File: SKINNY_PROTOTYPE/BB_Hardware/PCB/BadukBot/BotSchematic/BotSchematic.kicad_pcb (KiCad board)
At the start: 2 copper layers, 68 parts, among them J1 MOLEX_78171-0002, J2 MOLEX_78171-0003, Q1 MMBT3904LT1G, Q2 MMBT3904LT1G, Q3 MMBT3904LT1G, Q4 MMBT3904LT1G, U1 STM32F051C8U6, U2 LSM6DS3, U3 A3901SEJTR-T, U4 ADP122ACPZ-3.3-R7, U5 AT42QT1070-MMHCT-ND, U6 MCP73831T-2ACI_OT, U7 NRF24L01P-R7, Y1 7V-16.000MAAE-T

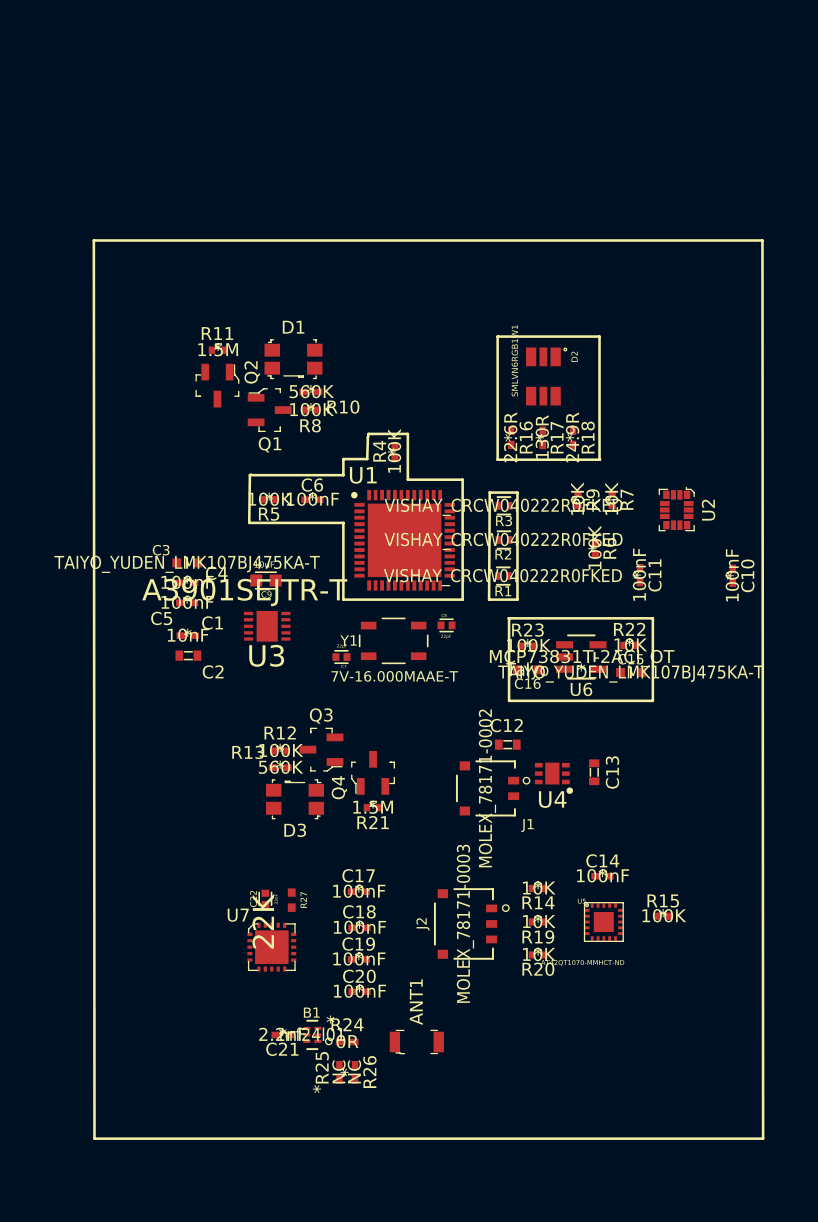
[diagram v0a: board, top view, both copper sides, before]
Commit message: PCB adjustments
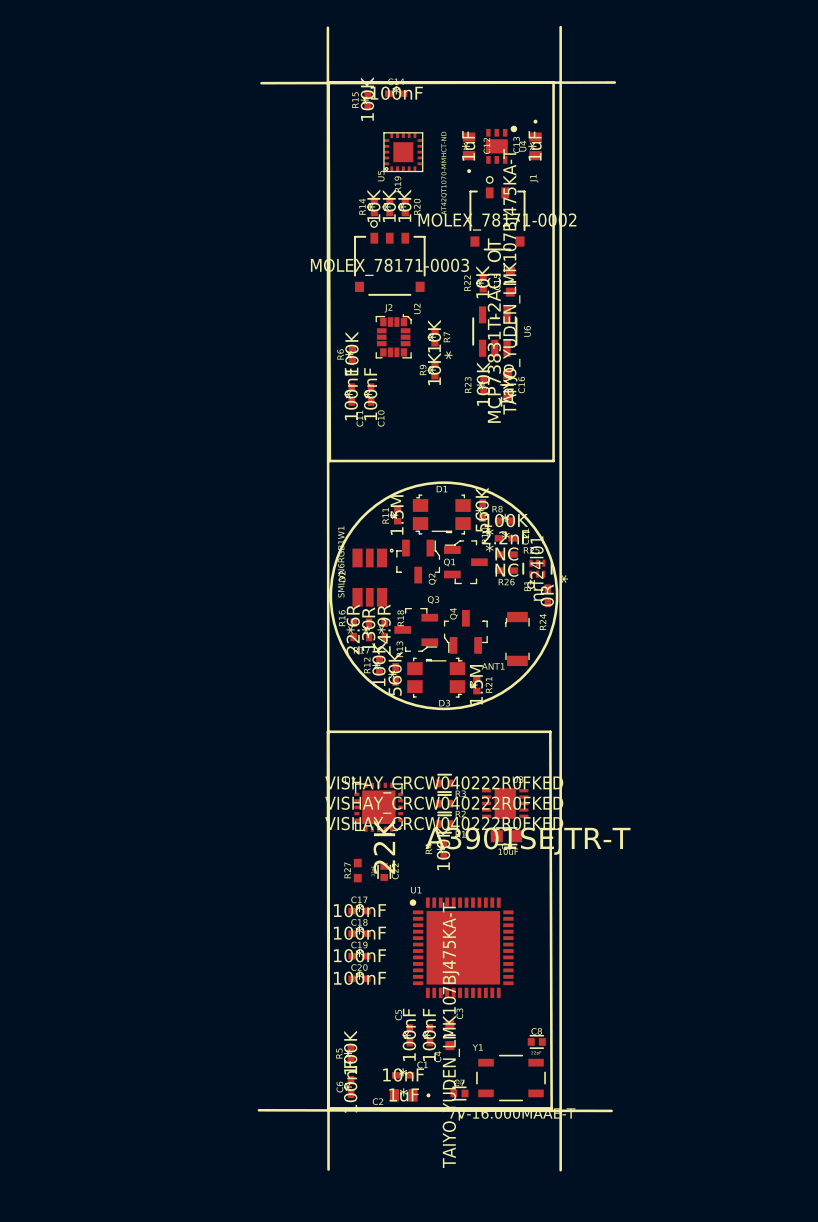
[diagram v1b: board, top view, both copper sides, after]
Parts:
- B1: footprint 2450BM14A0002T:JOHANSON_2450BM14A0002T_0 -> JOHANSON_2450BM14A0002T:JOHANSON_2450BM14A0002T_0
- C12, C13, C2: footprint digikey-footprints:0603 -> 1uF:0603ZD105KAT2A
- C22: footprint 22pf_GRM1555C1H220JA01D:CAPC1005X55N -> 33nF:CAPC1005X55N
- C9: footprint 100uF:CAPC1608X9N -> 10uF:CAPC1608X9N
- moved R15 67.3 mm to (216.5, 71.3), turned to 90 degrees
- moved C14 62.8 mm to (218.7, 70.8)
- moved U5 61.7 mm to (219.2, 75.3), turned to 90 degrees
- moved R20 58.9 mm to (219.3, 79.5), turned to 270 degrees
- moved R19 56.6 mm to (218.1, 79.5), turned to 270 degrees
- moved R14 54.4 mm to (216.9, 79.5), turned to 270 degrees
- moved J2 51.4 mm to (218.2, 84.1), turned to 0 degrees
- moved U4 48.8 mm to (226.4, 74.8), turned to 270 degrees
- moved C13 48.8 mm to (229.4, 74.8), turned to 270 degrees
- moved C12 46.5 mm to (224.3, 74.8), turned to 90 degrees
- moved C6 45.6 mm to (215.2, 147.8), turned to 270 degrees
- moved J1 44.1 mm to (226.5, 80.6), turned to 0 degrees
- moved R5 43.4 mm to (215.2, 145.2), turned to 90 degrees
- moved C21 42.2 mm to (227.2, 105.2)
- moved R25 42.2 mm to (227.2, 106.5), turned to 180 degrees
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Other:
- copper layers 2 -> 4
